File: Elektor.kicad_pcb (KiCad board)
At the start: 2 copper layers, 54 parts, among them J1 Conn_Coaxial, J13 Conn_Coaxial, J6 Conn_01x03_Pin, J7 Conn_01x02, J8 Conn_01x02, Q1 BF545B, U1 Si5351A-B-GT, U2 74HC74, U3 74HC4066D_653, U5 MCP6022, U6 AUDIOSHIELD-REVD, U7 MCP6022, Y1 ABM7-25.000MHZ-D2Y-T

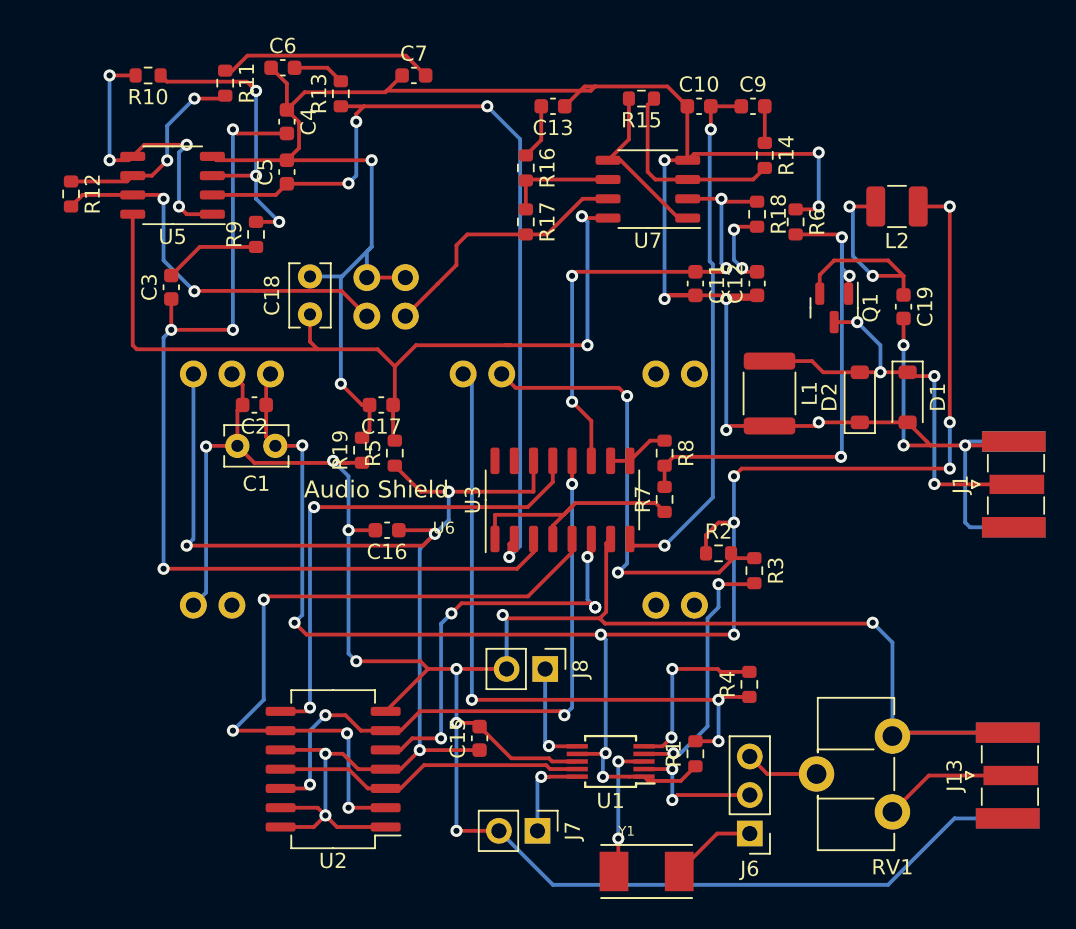
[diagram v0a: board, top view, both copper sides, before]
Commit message: routage plus compact
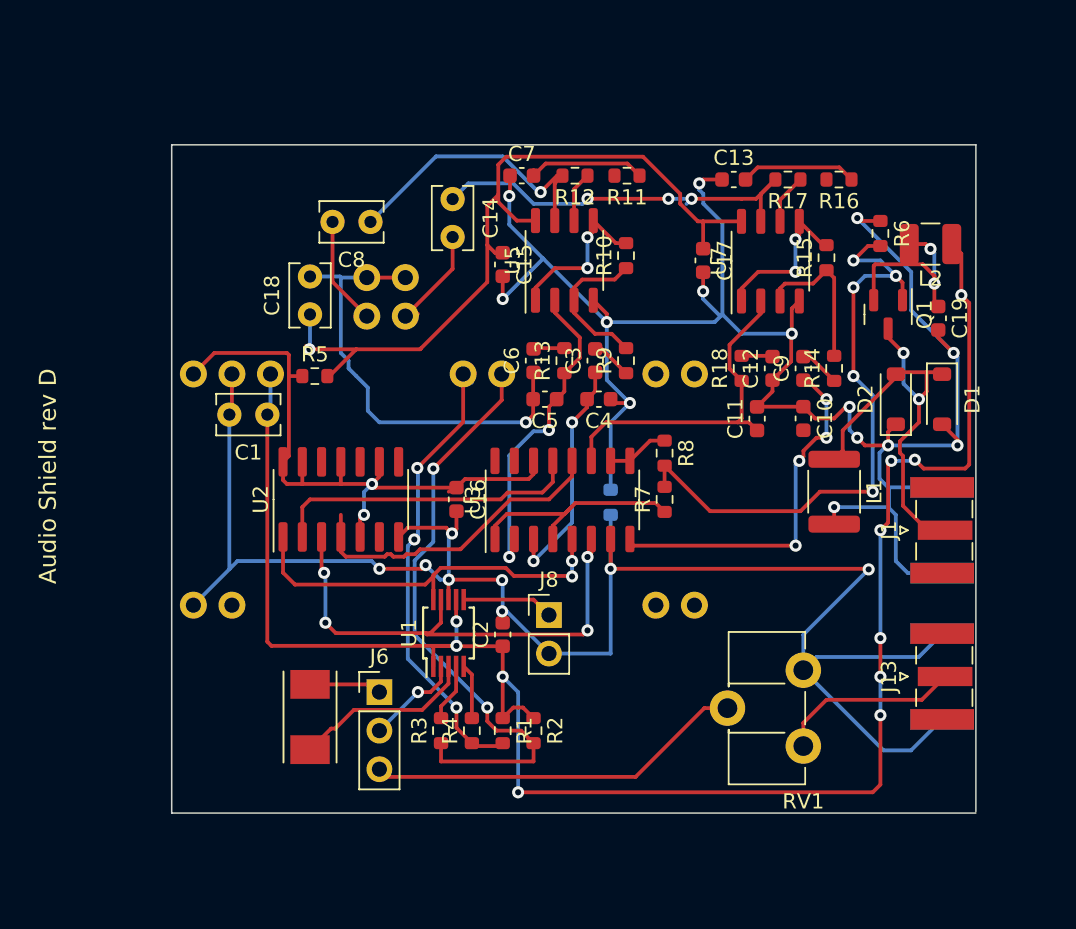
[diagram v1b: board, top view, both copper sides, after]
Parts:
- removed J7: Conn_01x02, Connector_PinHeader_2.54mm:PinHeader_1x02_P2.54mm_Vertical
- added C14: 4.7u, Capacitor_THT:C_Rect_L4.0mm_W2.5mm_P2.50mm, F.Cu at (175.5, 64.5)
- added C8: 4.7u, Capacitor_THT:C_Rect_L4.0mm_W2.5mm_P2.50mm, F.Cu at (170.1, 66.0)
- R19: moved to B.Cu
- U2: value 74HC74 -> 74HC04; footprint Package_SO:SO-14_5.3x10.2mm_P1.27mm -> Package_SO:SOIC-14_3.9x8.7mm_P1.27mm
- moved R10 33.7 mm to (186.9, 68.3), turned to 90 degrees
- moved R12 33.2 mm to (183.6, 63.0), turned to 180 degrees
- moved C15 31.3 mm to (178.8, 68.8), turned to -90 degrees
- moved C3 28.4 mm to (184.9, 75.2)
- moved C4 27.5 mm to (185.2, 77.7), turned to 180 degrees
- moved R11 27.2 mm to (187.0, 63.0), turned to 180 degrees
- moved U5 26.3 mm to (182.9, 68.6), turned to 90 degrees
- moved J6 26.1 mm to (170.7, 97.0), turned to 0 degrees
- moved R9 25.8 mm to (186.9, 75.2)
- moved C6 25.4 mm to (180.8, 75.2), turned to 90 degrees
- moved Y1 24.4 mm to (166.1, 98.7), turned to 90 degrees
- moved C17 23.2 mm to (192.0, 68.6), turned to -90 degrees
- moved R3 23.2 mm to (174.8, 99.6), turned to 90 degrees
- moved R13 22.9 mm to (182.9, 75.2)
- moved C5 22.7 mm to (181.6, 77.7), turned to 180 degrees
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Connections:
- C15 pad 1: Net-(U2A-~{R}) -> 5VA
- C15 pad 2: GND -> GNDA
- C16 pad 1: Net-(U2A-~{R}) -> Net-(U2G-VCC)
- R12 pad 2: Net-(R12-Pad2) -> Net-(C8-Pad1)
- R17 pad 2: Net-(R17-Pad2) -> Net-(C14-Pad1)
- R5 pad 1: Net-(U2A-~{R}) -> Net-(U2G-VCC)
- U1 pad 10: Net-(J7-Pin_1) -> Net-(U1-CLK0)
- U2 pad 1: Net-(U2A-~{R}) -> Net-(U1-CLK0)
- U2 pad 10: Net-(U2A-~{R}) -> unconnected-(U2-Pad10)
- U2 pad 11: Net-(U1-CLK1) -> Net-(U2G-VCC)
- U2 pad 12: Net-(U2A-~{Q}) -> unconnected-(U2-Pad12)
- U2 pad 13: Net-(U2A-~{R}) -> Net-(U2G-VCC)
- U2 pad 14: Net-(U2A-~{R}) -> Net-(U2G-VCC)
- U2 pad 2: Net-(U2A-D) -> Net-(U3-1E)
- U2 pad 4: Net-(U2A-~{R}) -> Net-(U3-4E)
- U2 pad 5: Net-(U2A-Q) -> Net-(U2G-VCC)
- U2 pad 6: Net-(U2A-~{Q}) -> unconnected-(U2-Pad6)
- U2 pad 8: Net-(U2B-~{Q}) -> unconnected-(U2-Pad8)
- U2 pad 9: Net-(U2A-D) -> Net-(U2G-VCC)
- U3 pad 12: Net-(U2A-~{Q}) -> Net-(U3-4E)
- U3 pad 13: Net-(U2B-~{Q}) -> Net-(U3-1E)
- U3 pad 14: Net-(U2A-~{R}) -> Net-(U2G-VCC)
- U3 pad 5: Net-(U2A-D) -> Net-(U1-CLK0)
- U3 pad 6: Net-(U2A-Q) -> Net-(U1-CLK1)
- U5 pad 7: Net-(R12-Pad2) -> Net-(C8-Pad1)
- U6 pad 5V: Net-(U2A-~{R}) -> Net-(U2G-VCC)
- U6 pad INL: Net-(R12-Pad2) -> Net-(C8-Pad2)
- U6 pad INR: Net-(R17-Pad2) -> Net-(C14-Pad2)
- U7 pad 7: Net-(R17-Pad2) -> Net-(C14-Pad1)
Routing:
- net Net-(U2A-~{R}): track 89.3 -> 0.00 mm, vias 6 -> 0
- net GND: track 174.0 -> 115.5 mm, vias 9 -> 8
- net Net-(U3-2Z): track 64.6 -> 16.4 mm, vias 4 -> 2
- net Net-(U2A-D): track 47.2 -> 0.00 mm, vias 4 -> 0
- net Net-(U2G-VCC): track 0.00 -> 42.6 mm, vias 0 -> 2
- net Net-(U2A-~{Q}): track 40.8 -> 0.00 mm, vias 4 -> 0
- net Net-(U3-1Z): track 56.7 -> 20.1 mm, vias 4 -> 2
- net Net-(U2B-~{Q}): track 33.2 -> 0.00 mm, vias 2 -> 0
- net Net-(U2A-Q): track 27.2 -> 0.00 mm, vias 5 -> 0
- net Net-(C14-Pad1): track 0.00 -> 26.6 mm, vias 0 -> 3
- net Net-(U1-CLK0): track 0.00 -> 26.5 mm, vias 0 -> 2
- net Net-(R12-Pad2): track 25.5 -> 0.00 mm, vias 2 -> 0
- net Net-(U3-4E): track 0.00 -> 21.2 mm
- net Net-(U3-1E): track 0.00 -> 20.6 mm
- net Net-(J6-Pin_3): track 4.88 -> 25.0 mm
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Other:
- board outline added: 53 x 44 mm
